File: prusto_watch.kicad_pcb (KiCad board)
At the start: 2 copper layers, 56 parts, among them J1 USB_microB_2040002-1, J2 Conn_02x05_Odd_Even, J3 Vibration Motor, J4 Conn_01x06, J5 Conn_01x08, J6 Conn_02x03_Odd_Even, J7 Conn_02x03_Counter_Clockwise, J8 Screw_Terminal_01x01, J9 Screw_Terminal_01x01, Q3 RUM002N02T2L, SW2 SW_Push, U1 STM32F303RCT6-48, U2 LTC4063, U3 LIS3DETR, U5 TPS60241DGKR, U7 RT9818A-18GV, U8 WM1389CT-ND, Y1 ECS.327, Y2 FA-238

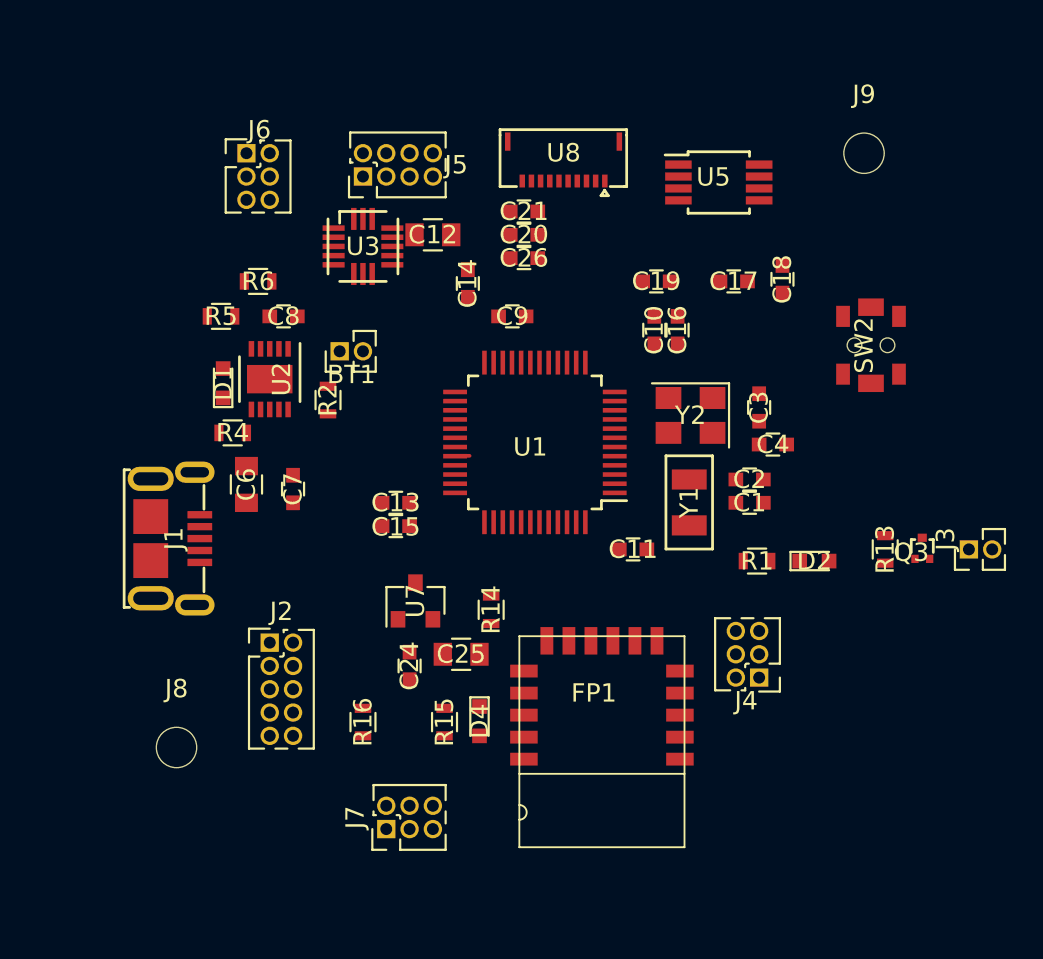
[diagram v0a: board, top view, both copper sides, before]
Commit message: Finalize Routing
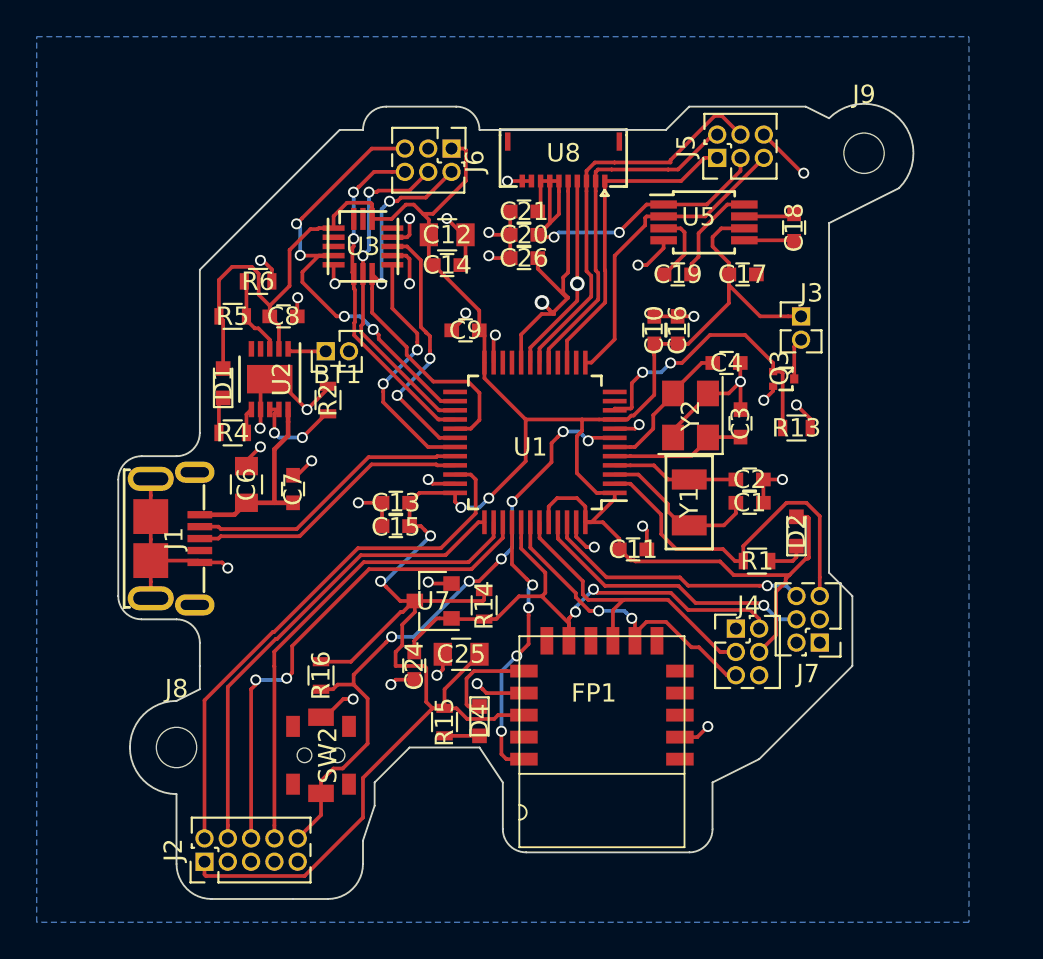
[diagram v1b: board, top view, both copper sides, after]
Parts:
- J5: value Conn_01x08 -> Conn_01x06; footprint Pin_Headers:Pin_Header_Straight_2x04_Pitch1.27mm -> Pin_Headers:Pin_Header_Straight_2x03_Pitch1.27mm
- moved SW2 37.4 mm to (134.9, 115.4), turned to 270 degrees
- moved J7 25.7 mm to (162.1, 109.2), turned to 180 degrees
- moved J5 19.3 mm to (156.5, 82.8)
- moved J3 15.6 mm to (161.0, 91.4), turned to 0 degrees
- moved J2 12.5 mm to (128.5, 121.2), turned to 90 degrees
- moved J6 11.2 mm to (142.0, 82.3), turned to 270 degrees
- moved Q3 11.1 mm to (160.7, 94.8), turned to 270 degrees
- moved R13 8.20 mm to (160.8, 97.5), turned to 0 degrees
- moved C4 5.11 mm to (157.0, 94.0), turned to 0 degrees
- moved R16 3.42 mm to (134.9, 111.0), turned to 270 degrees
- moved J4 2.95 mm to (157.5, 108.5), turned to 0 degrees
- moved C18 2.89 mm to (160.7, 86.6)
- moved C9 2.66 mm to (142.7, 92.2), turned to 180 degrees
- moved U5 2.32 mm to (155.7, 86.3)
- moved D2 1.89 mm to (160.8, 103.2), turned to 90 degrees
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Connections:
- J4 pad 1: +3V3 -> (no net)
- J4 pad 2: /RX_BLE -> /BLE_nRST
- J4 pad 4: /BLE_CONF -> +3V3
- J4 pad 5: /BLE_nRST -> /RX_BLE
- J5 pad 1: +5V -> /DISP_SCLK
- J5 pad 2: /DISP_EN -> /DISP_SDI
- J5 pad 3: /DISP_SCS -> +5V
- J5 pad 4: /DISP_SDI -> /DISP_SCS
- J5 pad 5: /DISP_SCLK -> /5V_EN
- J5 pad 6: /EXTCOMIN -> GND
- J6 pad 2: /ACC_SCK -> /ACC_CS
- J6 pad 3: /ACC_CS -> GND
- J6 pad 4: /ACC_SDI -> /ACC_SDO
- J6 pad 5: GND -> /ACC_SCK
- J6 pad 6: /ACC_SDO -> /ACC_SDI
- J7 pad 4: (no net) -> /BUTTON1
- J7 pad 5: (no net) -> /LED_1
- J7 pad 6: /BUTTON1 -> /BUTTON2
- U1 pad 11: /5V_EN -> (no net)
- U1 pad 12: /DISP_SCS -> (no net)
- U1 pad 13: /DISP_EN -> /5V_EN
- U1 pad 18: (no net) -> /DISP_SCS
- U1 pad 19: (no net) -> /EXTCOMIN
- U1 pad 20: (no net) -> /DISP_EN
- U1 pad 46: /EXTCOMIN -> /BUTTON2
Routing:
- net +3V3: track 0.00 -> 170.3 mm, vias 0 -> 4
- net GND: track 0.00 -> 83.6 mm, vias 0 -> 34
- net /STM_NRST: track 0.00 -> 35.1 mm, vias 0 -> 6
- net /BLE_nRST: track 0.00 -> 29.9 mm, vias 0 -> 2
- net /TMS: track 0.00 -> 29.6 mm
- net /TDO: track 0.00 -> 27.1 mm, vias 0 -> 2
- net /TCK: track 0.00 -> 26.0 mm
- net /TDI: track 0.00 -> 25.5 mm
- net /ACC_SCK: track 0.00 -> 25.0 mm, vias 0 -> 4
- net +5V: track 0.00 -> 22.7 mm, vias 0 -> 2
- net /ACC_CS: track 0.00 -> 22.5 mm, vias 0 -> 2
- net /DISP_SCS: track 0.00 -> 21.9 mm
- net /LED_1: track 0.00 -> 20.0 mm
- net /DISP_SDI: track 0.00 -> 19.0 mm
- net /ACC_SDI: track 0.00 -> 18.6 mm, vias 0 -> 2
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- added copper zone on B.Cu, net GND
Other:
- board outline added: 43.3 x 43.3 mm
